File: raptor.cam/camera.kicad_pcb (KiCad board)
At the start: 2 copper layers, 2 parts, among them P1 CONN_01X15, P2 FFC_FPC_connector_01X15

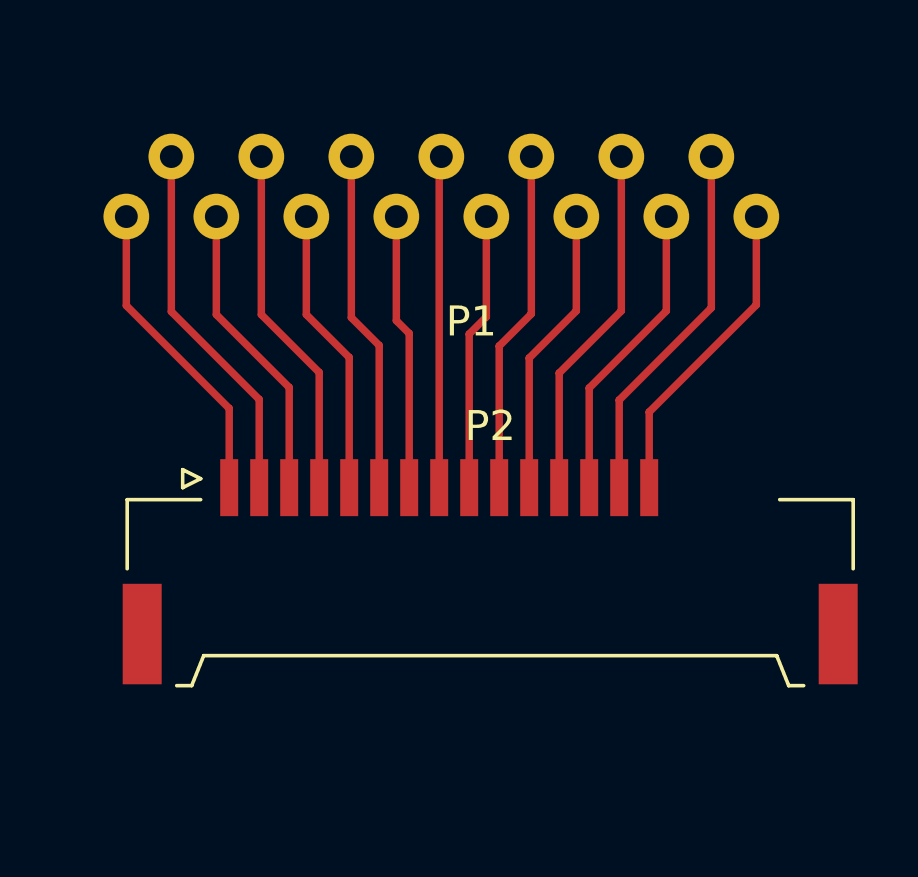
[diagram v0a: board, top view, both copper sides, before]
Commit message: Kamera cd.
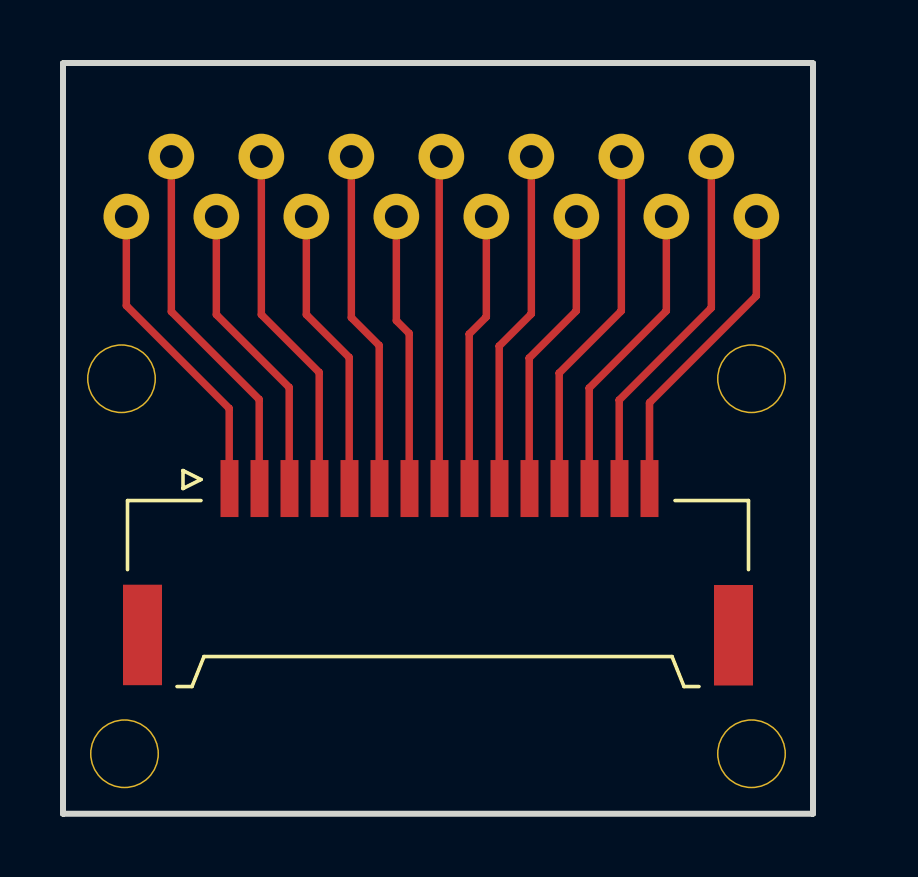
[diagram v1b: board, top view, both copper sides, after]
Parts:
- removed P2: FFC_FPC_connector_01X15, rpi:FFC_connector_15x1.0mm
- added ?: , rpi:FFC_connector_15x1.0mm, F.Cu at (148.0, 115.6)
- added ?: , rpi:2.20mmDrill, F.Cu at (137.6, 122.0)
- added ?: , rpi:2.20mmDrill, F.Cu at (158.5, 109.5)
- added ?: , rpi:2.20mmDrill, F.Cu at (158.5, 122.0)
- added ?: , rpi:2.20mmDrill, F.Cu at (137.5, 109.5)
- ?: renamed from P1; value CONN_01X15 -> (none)
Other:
- board outline added: 25 x 25 mm
